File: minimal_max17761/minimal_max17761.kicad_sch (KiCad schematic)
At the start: 24 parts, among them J1 FW-02-03-G-D-085-155, J2 FW-02-03-G-D-085-155, U1 MAX17761ATC+

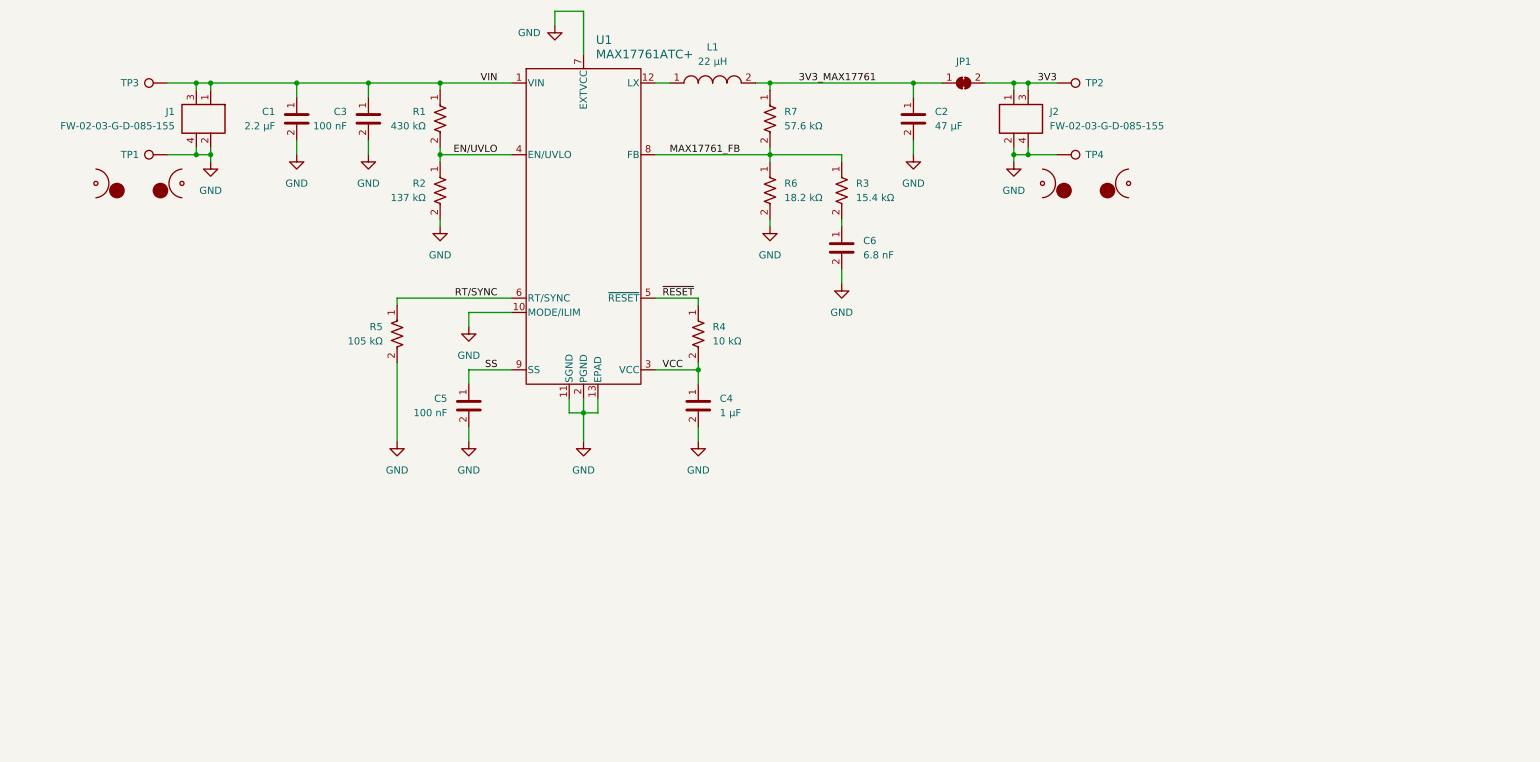
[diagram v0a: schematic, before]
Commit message: Backup
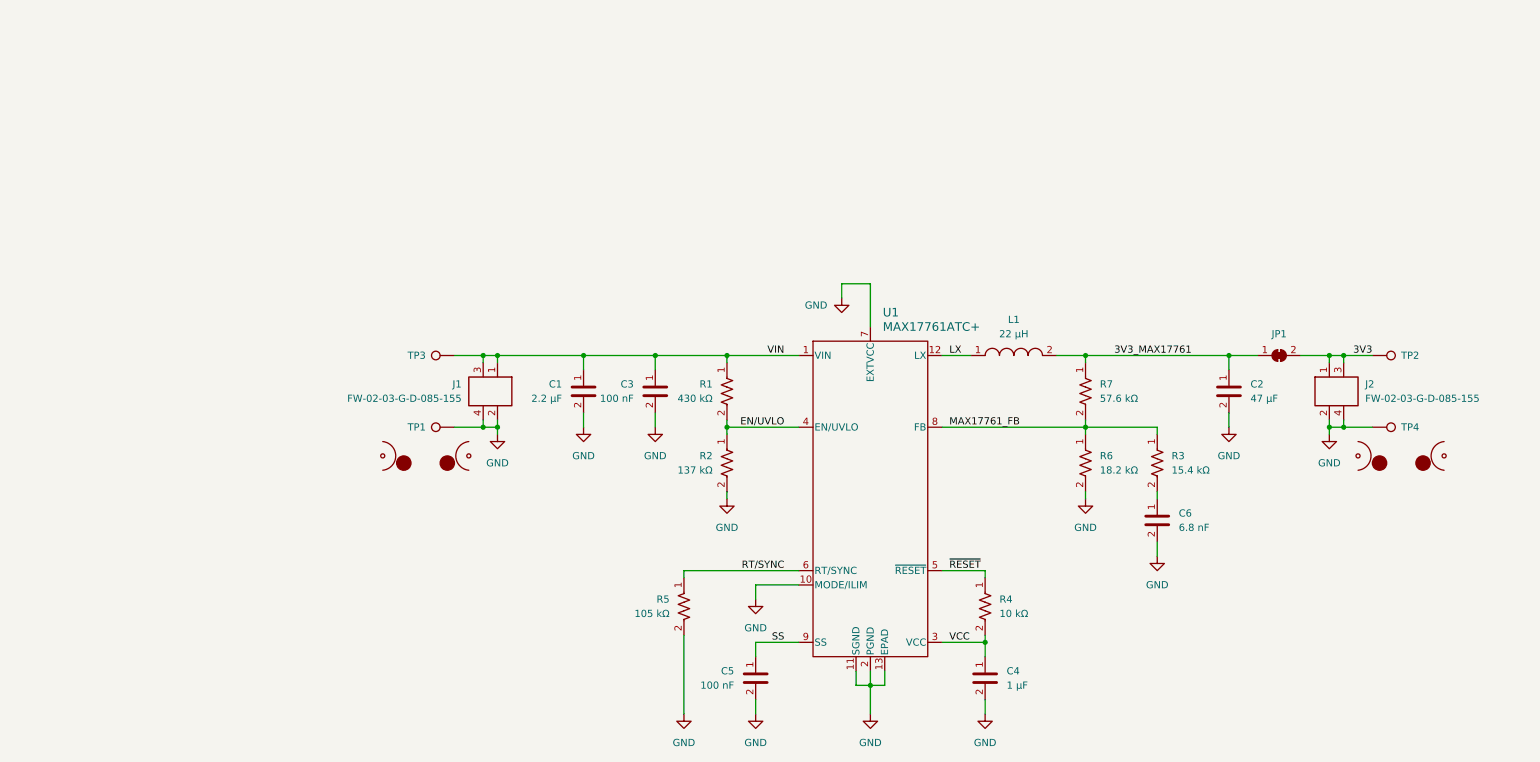
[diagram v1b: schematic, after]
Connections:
- net LX: now reaches L1.1, U1.12 (LX)
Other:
- moved on the sheet: C1, C2, C3, C4, C5, C6, J1, J2, JP1, L1, R1, R2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
